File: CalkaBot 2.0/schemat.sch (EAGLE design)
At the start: 55 parts, among them IC1 TB6612FNG, IC2 LM339D, IC3 7806DT, Q1 16MHz, X1 MINI-USB-32005-301

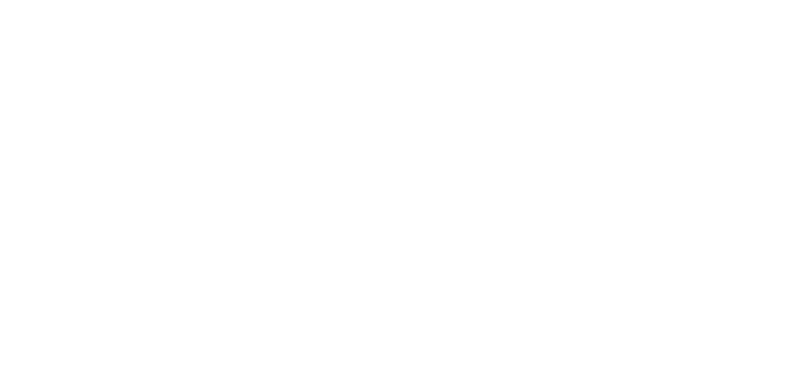
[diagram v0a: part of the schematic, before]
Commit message: niezapisane rzeczt
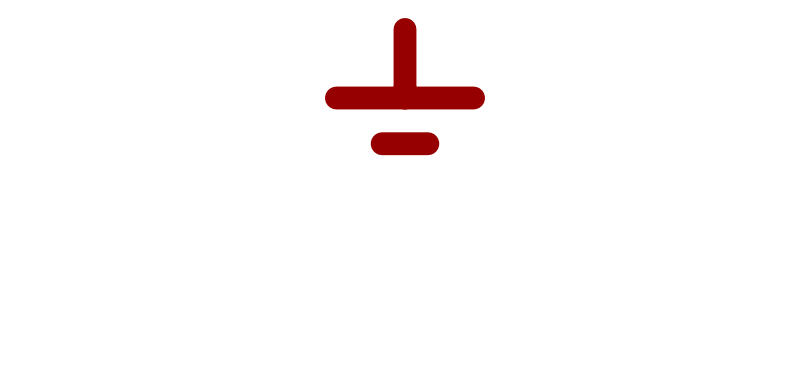
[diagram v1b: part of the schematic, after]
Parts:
- added U$3: (no value), untitled:GND
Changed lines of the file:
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@@
 <part name="P+3" library="supply1" library_urn="urn:adsk.eagle:library:371" deviceset="VCC" device=""/>
 <part name="GND2" library="supply1" library_urn="urn:adsk.eagle:library:371" deviceset="GND" device=""/>
-<part name="GND3" library="supply1" library_urn="urn:adsk.eagle:library:371" deviceset="GND" device=""/>
+<part name="GND3" library="supply1" library_urn="urn:adsk.eagle:library:371" deviceset="GND" device="">
+<attribute name="SPICEPREFIX" value="G"/>
+</part>
 <part name="R4" library="rcl" library_urn="urn:adsk.eagle:library:334" deviceset="R-EU_" device="R0805" package3d_urn="urn:adsk.eagle:package:23553/2" value="180R"/>
 <part name="P+4" library="supply1" library_urn="urn:adsk.eagle:library:371" deviceset="VCC" device=""/>
@@
 <part name="JP2" library="pinhead" library_urn="urn:adsk.eagle:library:325" deviceset="PINHD-1X5" device="" package3d_urn="urn:adsk.eagle:package:22469/2"/>
 <part name="JP3" library="pinhead" library_urn="urn:adsk.eagle:library:325" deviceset="PINHD-1X5" device="" package3d_urn="urn:adsk.eagle:package:22469/2"/>
+<part name="U$3" library="untitled" deviceset="GND" device=""/>
 </parts>
 <sheets>
@@
 <instance part="JP2" gate="A" x="-119.38" y="25.4" rot="R270"/>
 <instance part="JP3" gate="A" x="-119.38" y="15.24" rot="R270"/>
+<instance part="U$3" gate="G$1" x="-58.42" y="154.94"/>
 </instances>
 <busses>

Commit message: dodalem dipy
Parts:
- removed BUT1, BUT2, BUT3: (no value), switch-omron:10-XX
- removed JP3: (no value), pinhead:PINHD-1X5
- removed X1: MINI-USB-32005-301, con-cypressindustries:MINI-USB-32005-301
- added SW2: (no value), special:SW_DIP-3
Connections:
- removed net N$20: JP2.4, JP3.4, R26.1, X1.4
- new net N$11: JP2.4, R26.1
- net GND: now also SW2.4, SW2.5, SW2.6; no longer BUT1.S, BUT1.S1, BUT2.S, BUT2.S1, BUT3.S, BUT3.S1, JP3.1, JP3.2, X1.1, X1.2
- net MISO: now also SW2.3; no longer BUT1.P, BUT1.P1
- net MOSI: now also SW2.2; no longer BUT2.P, BUT2.P1
- net N$12: no longer JP3.3, X1.3
- net SCK: now also SW2.1; no longer BUT3.P, BUT3.P1
- net VBUS: no longer JP3.5, X1.5
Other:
- moved on the sheet: C10, R25, R26
